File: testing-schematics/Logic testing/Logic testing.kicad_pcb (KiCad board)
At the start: 2 copper layers, 79 x 76.8 mm, 47 parts, among them IC1 ESP32-C6-WROOM-1U-N8, J1 External Box, J2 Aux Wire, J3 Conn_01x04, J4 Lame Tab, J5 Test Output, K1 G6K-2, K2 G6K-2, K3 G6K-2, K4 G6K-2, K5 G6K-2, P1 USB_C_Plug_USB2.0, Q1 BC547, Q2 BC547, Q3 BC547, Q4 BC547, SW1 SW_SPDT, SW2 SW_DP3T, SW3 SW_Push, U2 AMS1117-3.3

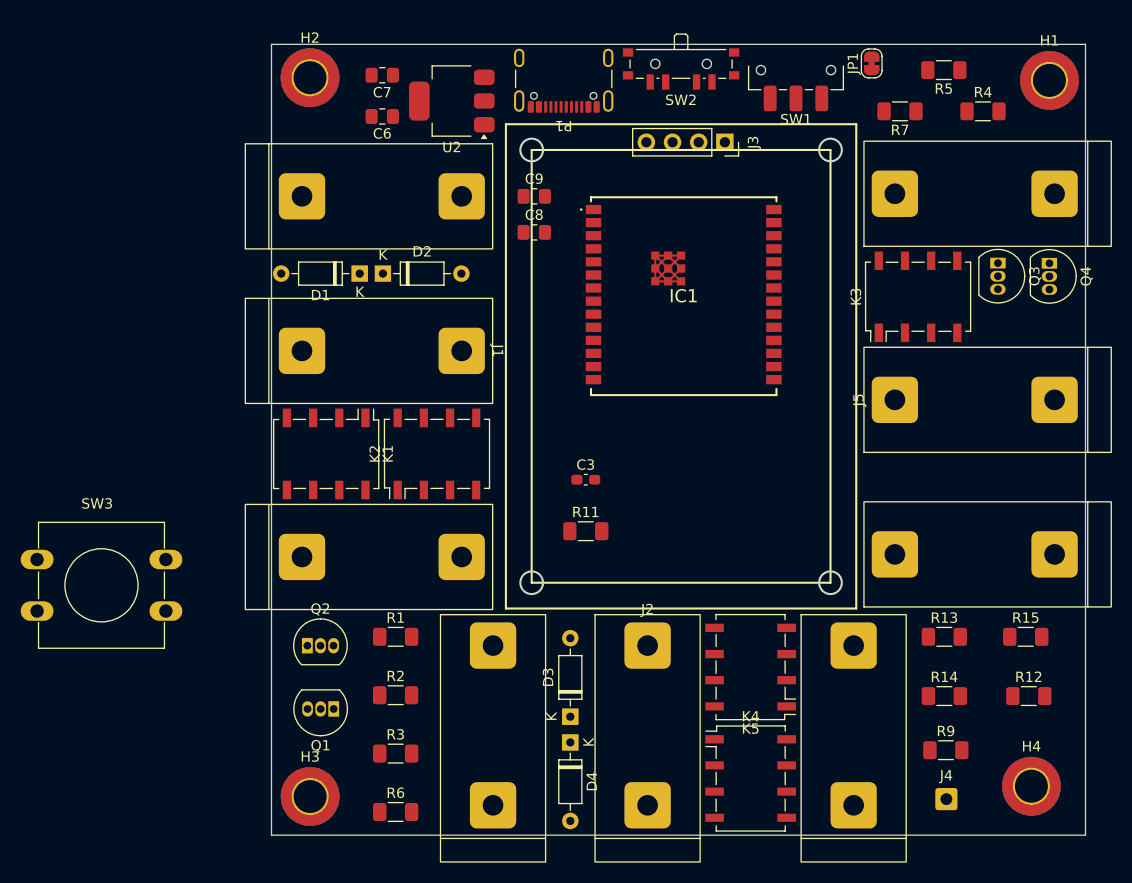
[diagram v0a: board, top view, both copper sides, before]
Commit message: Work from 14th
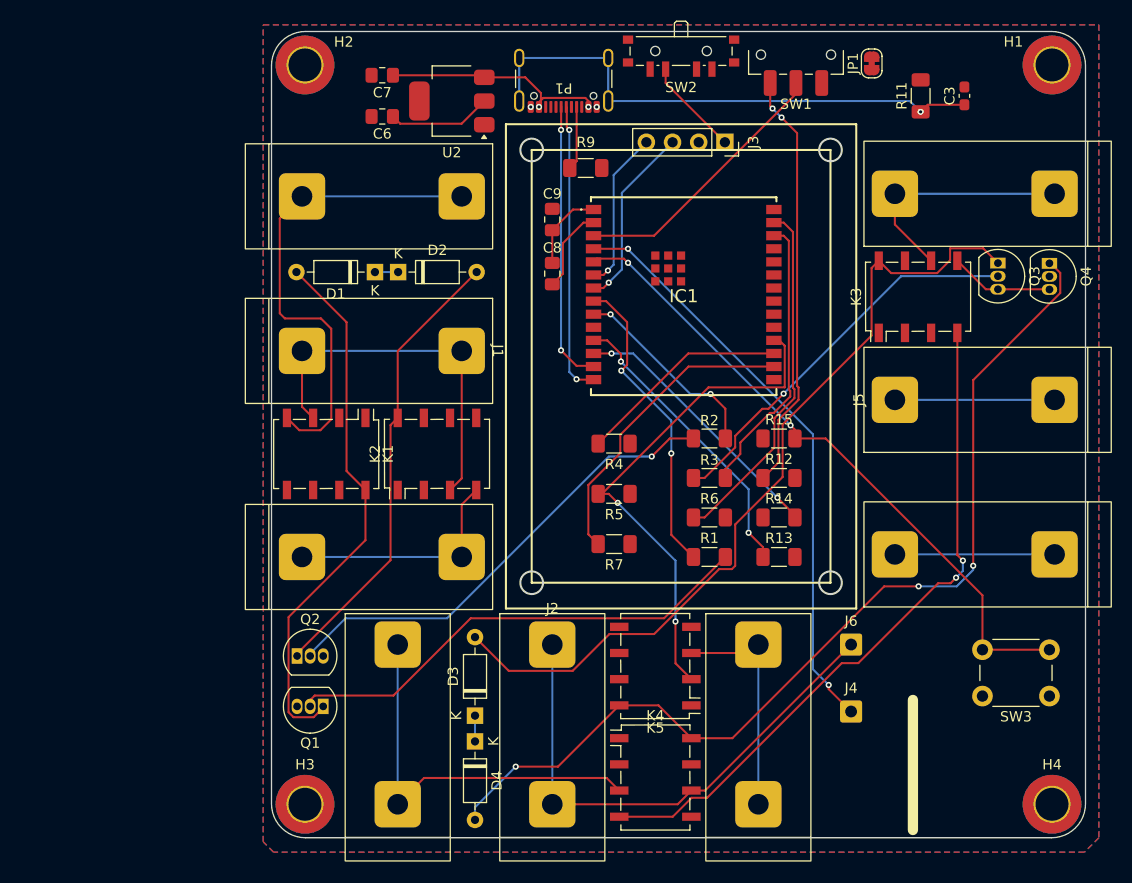
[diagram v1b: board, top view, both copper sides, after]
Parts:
- added J6: Small Pin, Connector_Wire:SolderWire-0.5sqmm_1x01_D0.9mm_OD2.1mm, F.Cu at (117.2, 106.8)
- SW3: footprint Button_Switch_THT:SW_PUSH-12mm -> Button_Switch_THT:SW_PUSH_6mm_H13mm
- moved SW3 99.1 mm to (136.5, 111.8), turned to 180 degrees
- moved R9 66.4 mm to (91.5, 60.5)
- moved R11 53.3 mm to (124.0, 53.5), turned to 90 degrees
- moved C3 52.3 mm to (128.2, 53.5), turned to 90 degrees
- moved R5 52.1 mm to (94.2, 92.1)
- moved R7 50.3 mm to (94.2, 97.0)
- moved R4 48.2 mm to (94.2, 87.2), turned to 180 degrees
- moved R6 41.8 mm to (103.5, 94.4)
- moved R3 40.5 mm to (103.5, 90.6), turned to 180 degrees
- moved R2 39.3 mm to (103.5, 86.8), turned to 180 degrees
- moved R12 32.2 mm to (110.2, 90.6)
- moved R1 31.4 mm to (103.5, 98.2)
- moved R15 30.7 mm to (110.2, 86.8)
- moved R14 23.6 mm to (110.2, 94.4)
- moved R13 17.8 mm to (110.2, 98.2)
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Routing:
- net Net-(D4-A): track 0.00 -> 95.5 mm, vias 0 -> 3
- net Net-(D3-A): track 0.00 -> 80.5 mm
- net SG1: track 0.00 -> 66.6 mm, vias 0 -> 2
- net BTN USE: track 0.00 -> 63.7 mm, vias 0 -> 2
- net LAME: track 0.00 -> 57.2 mm, vias 0 -> 2
- net Net-(D1-A): track 0.00 -> 52.7 mm
- net Net-(P1-SHIELD): track 0.00 -> 52.3 mm, vias 0 -> 1
- net B2: track 0.00 -> 50.9 mm
- net VDR3: track 0.00 -> 50.0 mm, vias 0 -> 2
- net A1: track 0.00 -> 47.4 mm
- net Net-(Q1-B): track 0.00 -> 46.7 mm
- net Net-(Q2-B): track 0.00 -> 46.1 mm, vias 0 -> 1
- net Net-(D2-A): track 0.00 -> 44.5 mm
- net Net-(SW1-C): track 0.00 -> 40.9 mm, vias 0 -> 2
- net B1: track 0.00 -> 38.6 mm
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- added copper zone on B.Cu, net VD1
- added copper zone on F.Cu, net VD1
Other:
- board size 79 x 76.8 mm -> 79 x 78.2 mm
